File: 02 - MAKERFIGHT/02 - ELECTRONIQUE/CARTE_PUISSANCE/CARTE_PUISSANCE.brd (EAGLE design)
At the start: 36.8 x 93.7 mm, 15 parts

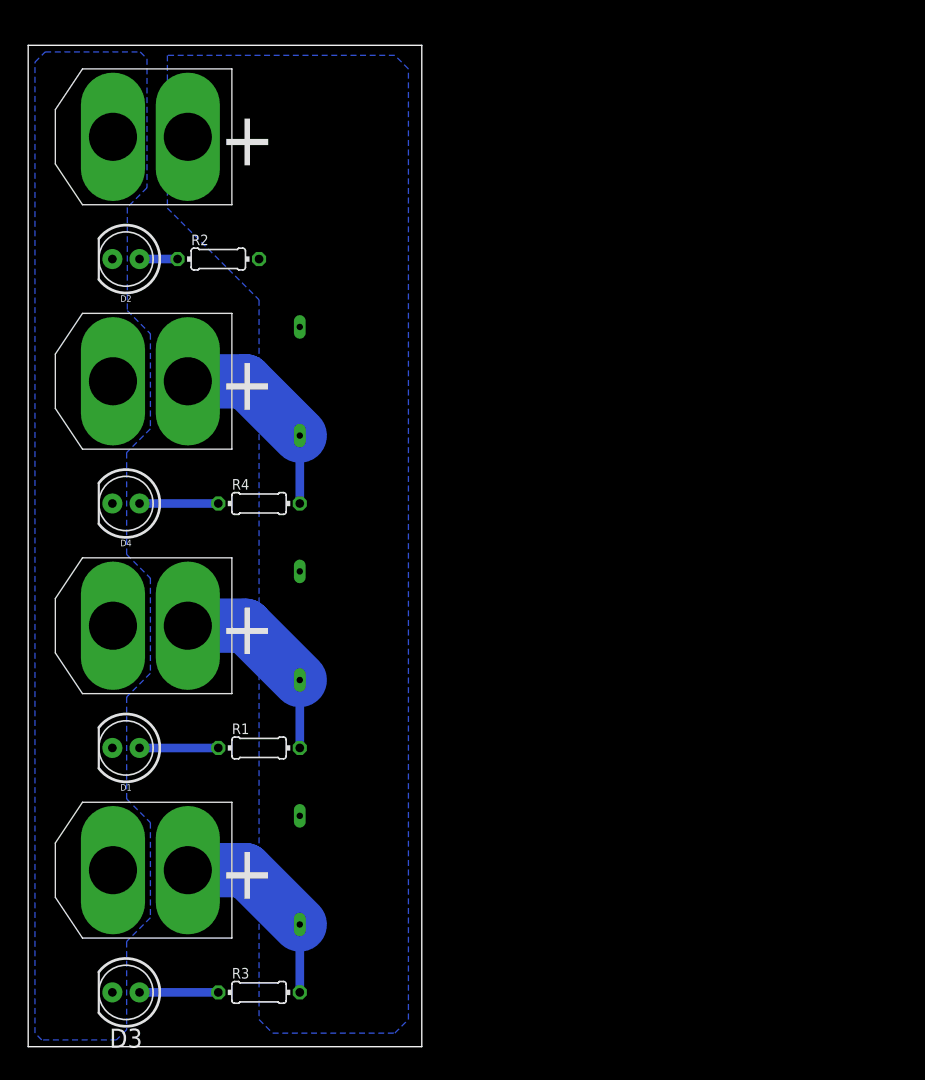
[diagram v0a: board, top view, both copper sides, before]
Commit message: update
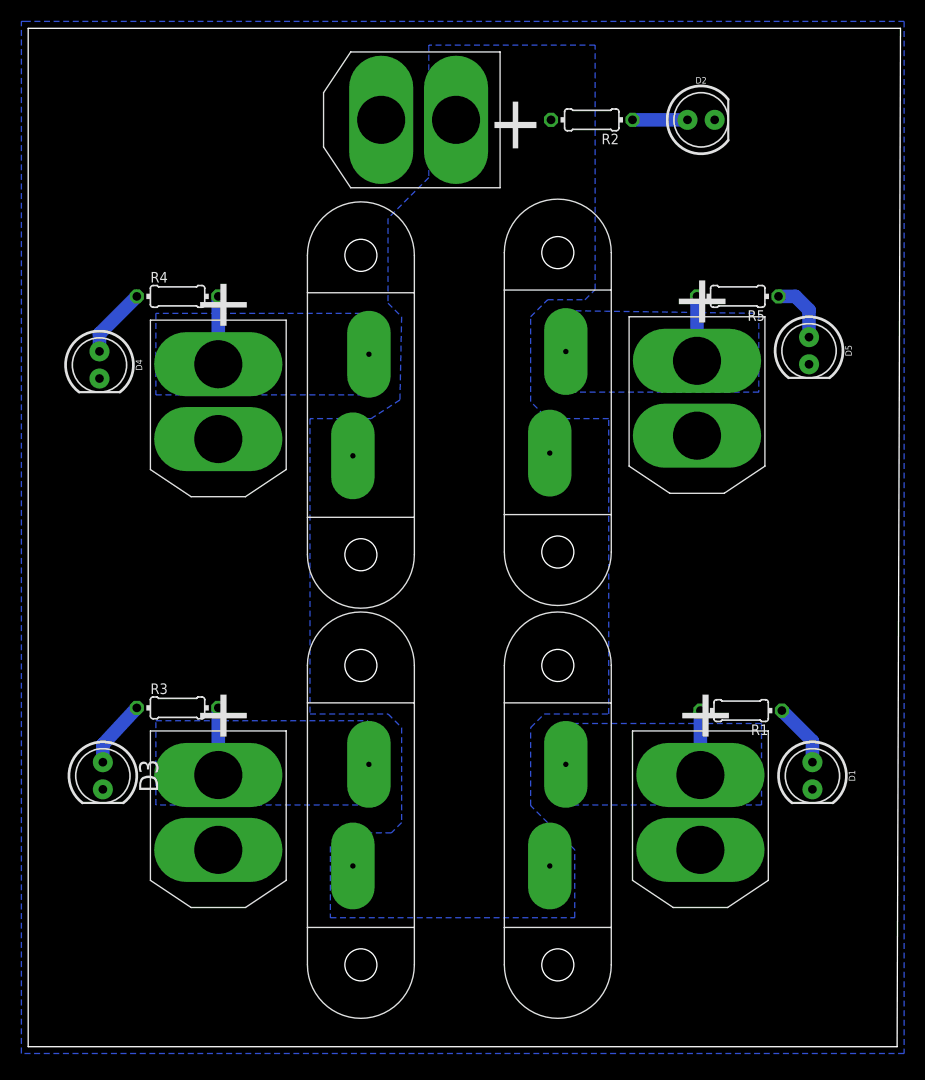
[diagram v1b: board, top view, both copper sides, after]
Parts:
- added D5: (no value), OPENBOT:LED_5MM
- added R5: (no value), rcl:0204/7
- added U$8: CONN_02_PUIXT60, OPENBOT:XT60
- added U$9: AUTOMOTIVE_FUSE, OPENBOT:AUTOMOTIVE_FUSE
- moved D1 64.3 mm to (73.3, 25.3), turned to 270 degrees
- moved D2 55.3 mm to (62.9, 86.7), turned to 0 degrees
- moved U$6 54.3 mm to (62.9, 21.9), turned to 270 degrees
- moved R1 45.2 mm to (66.7, 31.4), turned to 180 degrees
- moved R2 37.3 mm to (52.7, 86.7), turned to 180 degrees
- moved U$3 29.9 mm to (49.5, 21.7), turned to 90 degrees
- moved R3 27.7 mm to (14.0, 31.7)
- moved U$2 25.1 mm to (36.5, 86.7)
- moved R4 20.8 mm to (14.0, 70.2)
- moved D3 20.4 mm to (6.99, 25.3), turned to 270 degrees
- moved D4 13.2 mm to (6.67, 63.8), turned to 270 degrees
- moved U$4 8.33 mm to (17.8, 21.9), turned to 270 degrees
- moved U$5 7.69 mm to (31.1, 21.7), turned to 90 degrees
- moved U$7 6.63 mm to (17.8, 60.3), turned to 270 degrees
- moved U$1 6.13 mm to (31.1, 60.0), turned to 90 degrees
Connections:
- new net N$3: R5.2, U$8.P$1, U$9.P$2
- new net N$9: D5.A, R5.1
- net +12V: now also U$9.P$1
- net GND: now also D5.K, U$8.P$2
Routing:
- net N$1: track 18.9 -> 6.03 mm
- net N$5: track 18.9 -> 6.28 mm
- net N$7: track 18.6 -> 6.34 mm
- net N$3: track 0.00 -> 6.03 mm
- net N$9: track 0.00 -> 5.87 mm
- net N$4: track 3.56 -> 5.09 mm
- net N$2: track 7.37 -> 5.96 mm
- net N$6: track 7.37 -> 6.27 mm
- net N$8: track 7.37 -> 6.54 mm
- added copper zone on layer 16, net N$1
- added copper zone on layer 16, net N$3
- added copper zone on layer 16, net N$5
- added copper zone on layer 16, net N$7
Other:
- board size 36.8 x 93.7 mm -> 81.6 x 95.2 mm
